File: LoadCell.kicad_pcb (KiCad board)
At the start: 2 copper layers, 51.1 x 38.1 mm, 83 parts, among them J1 M20-8760242, J10 M20-8760242, J11 0.100_1X4, J12 0.100_1X4, J13 M20-8760242, J14 M20-8760242, J15 0.100_1X4, J16 0.100_1X4, J2 M20-8760242, J3 0.100_1X4, J4 0.100_1X4, J5 M20-8760242, J6 M20-8760242, J7 0.100_1X4, J8 0.100_1X4, J9 M20-8760242, U1 MCP6002, U2 MCP6002, U3 MCP6002, U4 MCP6002, U5 MCP6002, U6 MCP6002, U7 MCP6002, U8 MCP6002

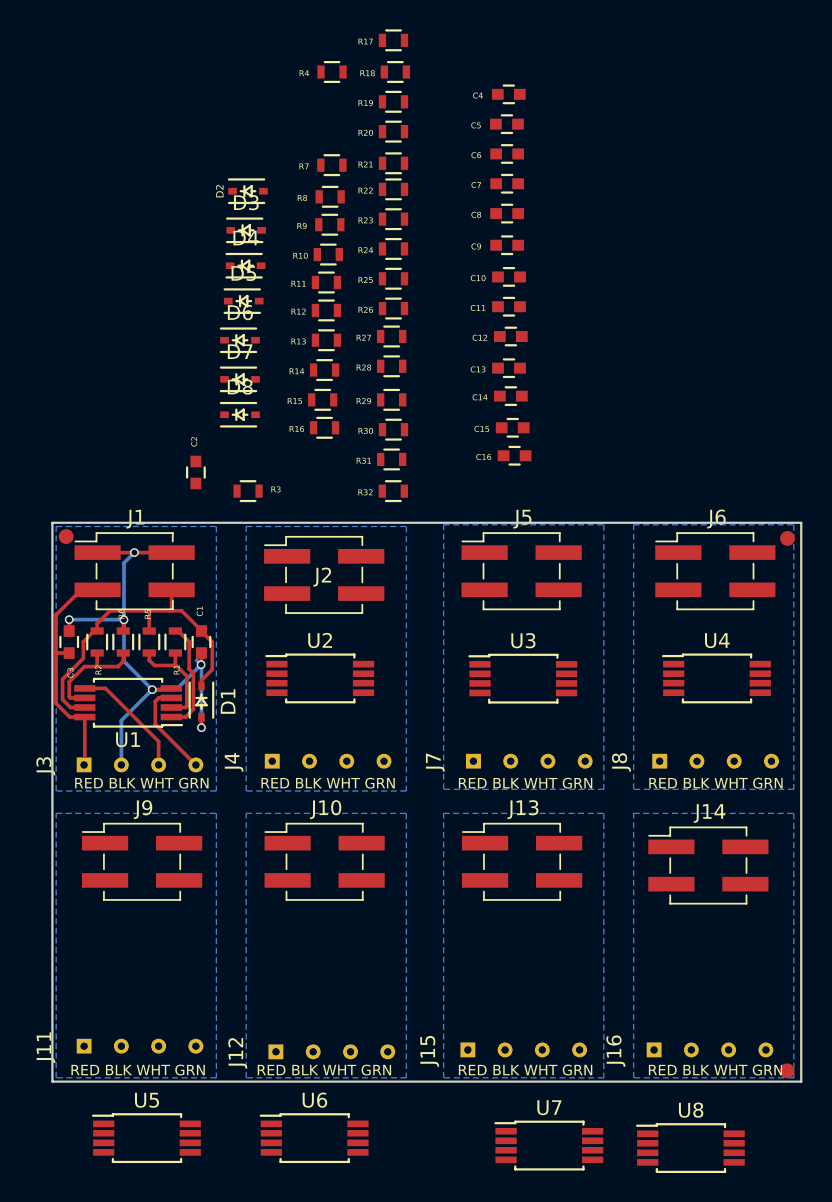
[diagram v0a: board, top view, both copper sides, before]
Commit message: Parts placed
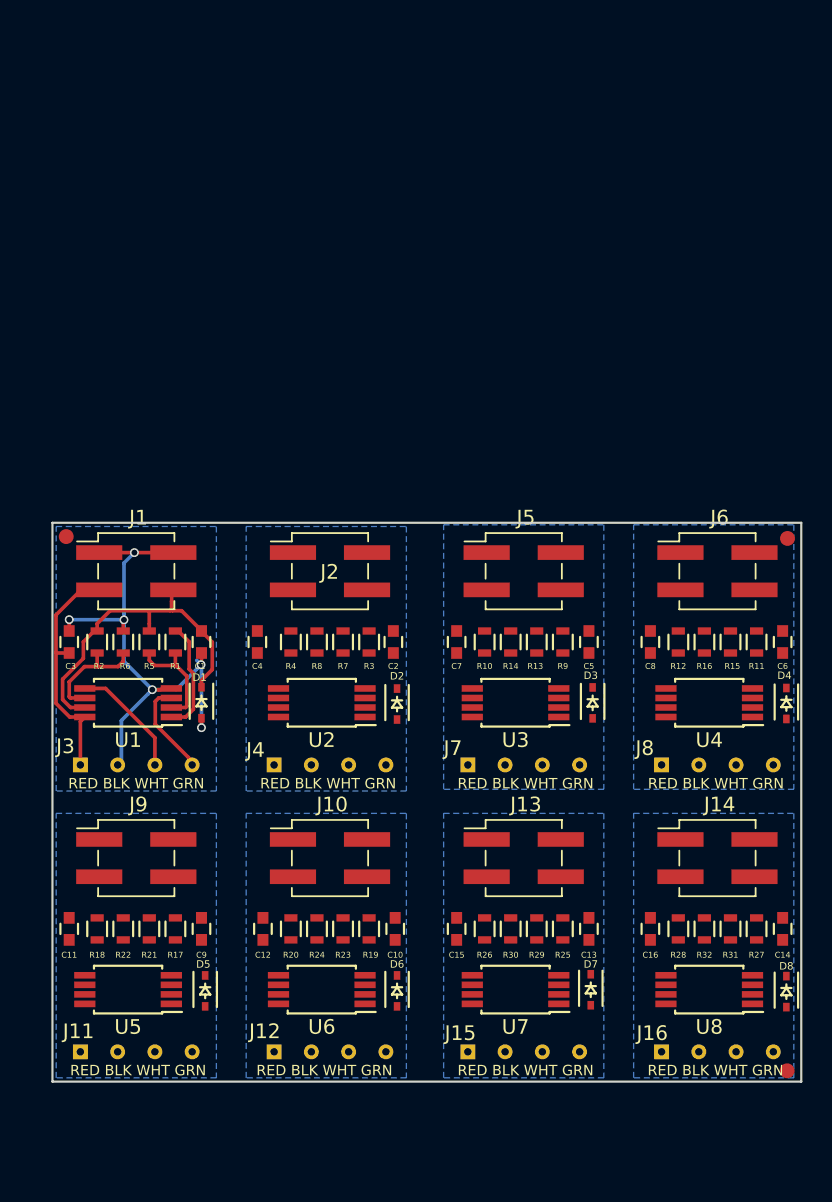
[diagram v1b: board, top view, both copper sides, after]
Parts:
- moved R17 62.4 mm to (110.0, 91.2), turned to 90 degrees
- moved R18 61.9 mm to (104.6, 91.2), turned to 90 degrees
- moved R19 56.4 mm to (123.2, 91.2), turned to 90 degrees
- moved R20 54.8 mm to (117.9, 91.2), turned to 90 degrees
- moved R21 54.8 mm to (108.2, 91.2), turned to 270 degrees
- moved D8 54.2 mm to (151.6, 95.5), turned to 270 degrees
- moved R22 53.7 mm to (106.4, 91.2), turned to 270 degrees
- moved C11 51.9 mm to (102.7, 91.2), turned to 90 degrees
- moved C9 51.1 mm to (111.8, 91.2), turned to 270 degrees
- moved R23 48.5 mm to (121.4, 91.2), turned to 270 degrees
- moved D7 48.0 mm to (138.3, 95.3), turned to 270 degrees
- moved D4 47.4 mm to (151.6, 75.8), turned to 270 degrees
- moved R27 47.4 mm to (149.6, 91.2), turned to 90 degrees
- moved D5 47.1 mm to (112.0, 95.4), turned to 270 degrees
- moved R24 46.6 mm to (119.6, 91.2), turned to 270 degrees
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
